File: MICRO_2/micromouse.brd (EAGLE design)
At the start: 100 x 80 mm, 27 parts

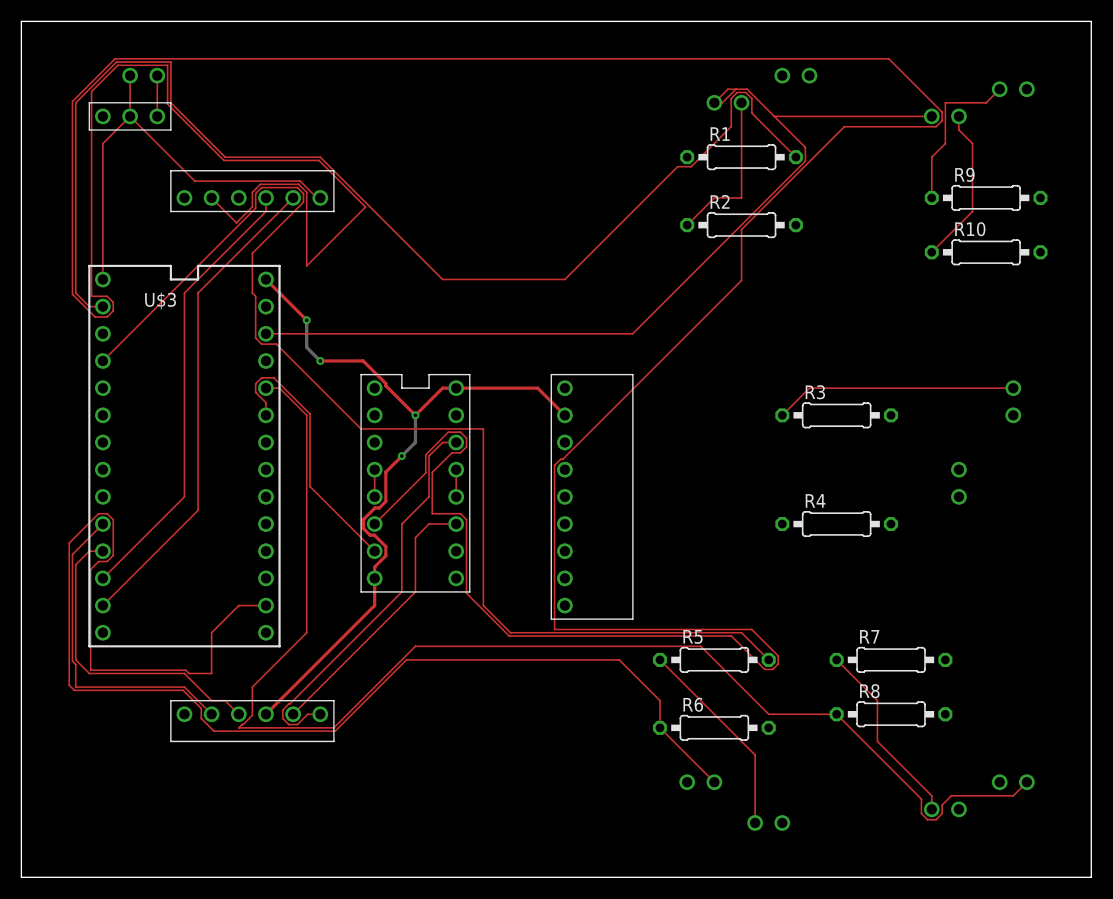
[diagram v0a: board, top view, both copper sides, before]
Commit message: Add files via upload
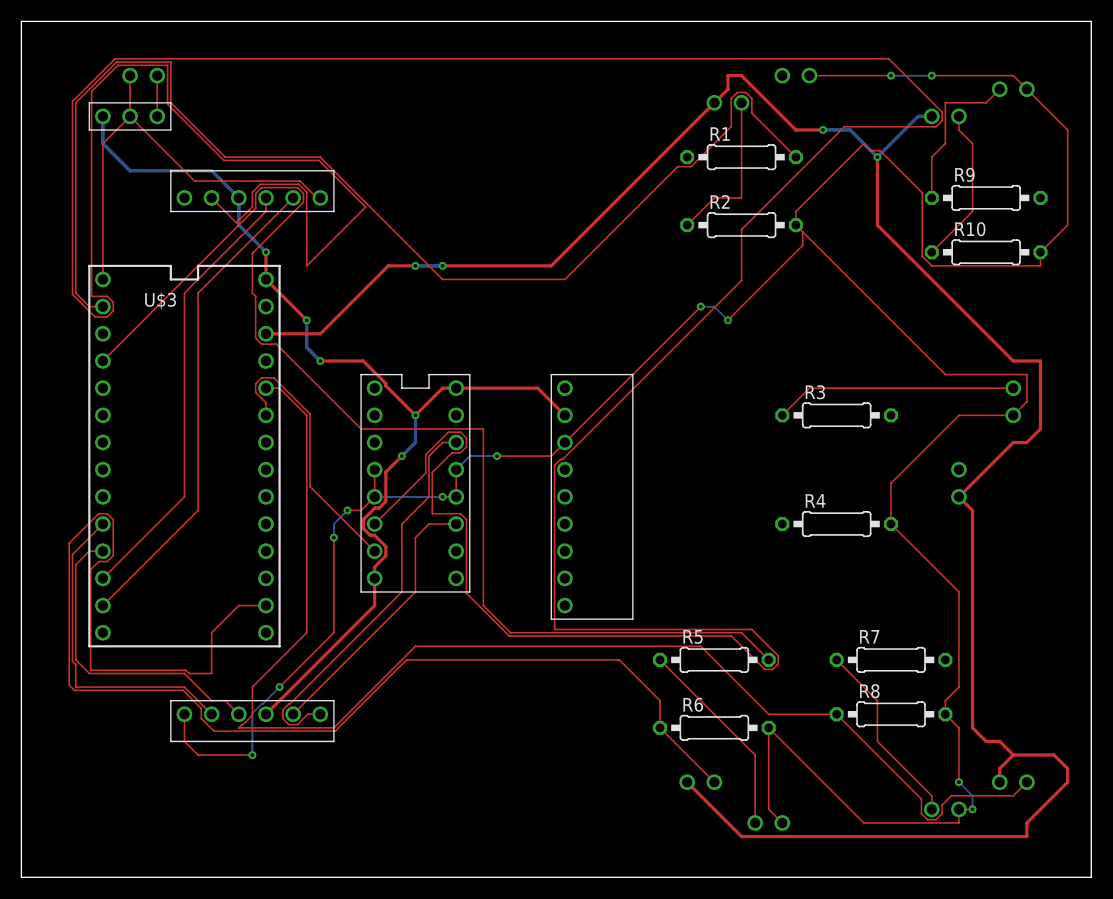
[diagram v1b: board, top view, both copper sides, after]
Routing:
- net GND: track 46.1 -> 325.0 mm, vias 0 -> 12
- net 3.3V_VCC: track 86.9 -> 198.6 mm, vias 0 -> 4
- net 5V_VCC: track 72.8 -> 98.9 mm, vias 4 -> 5
